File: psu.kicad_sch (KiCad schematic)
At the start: 10 parts, among them U2 TP6841

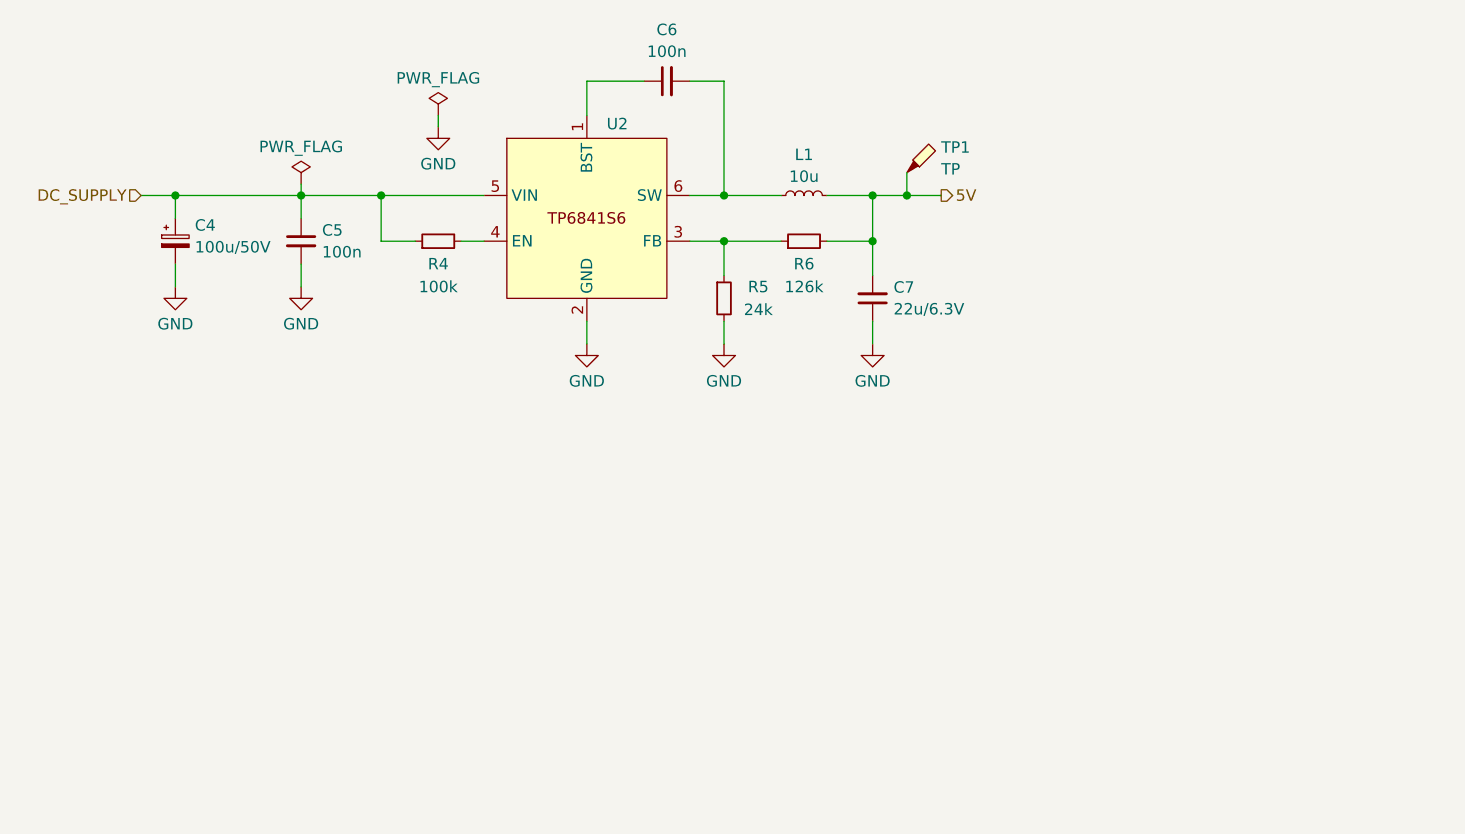
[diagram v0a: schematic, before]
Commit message: WIP PCB layout
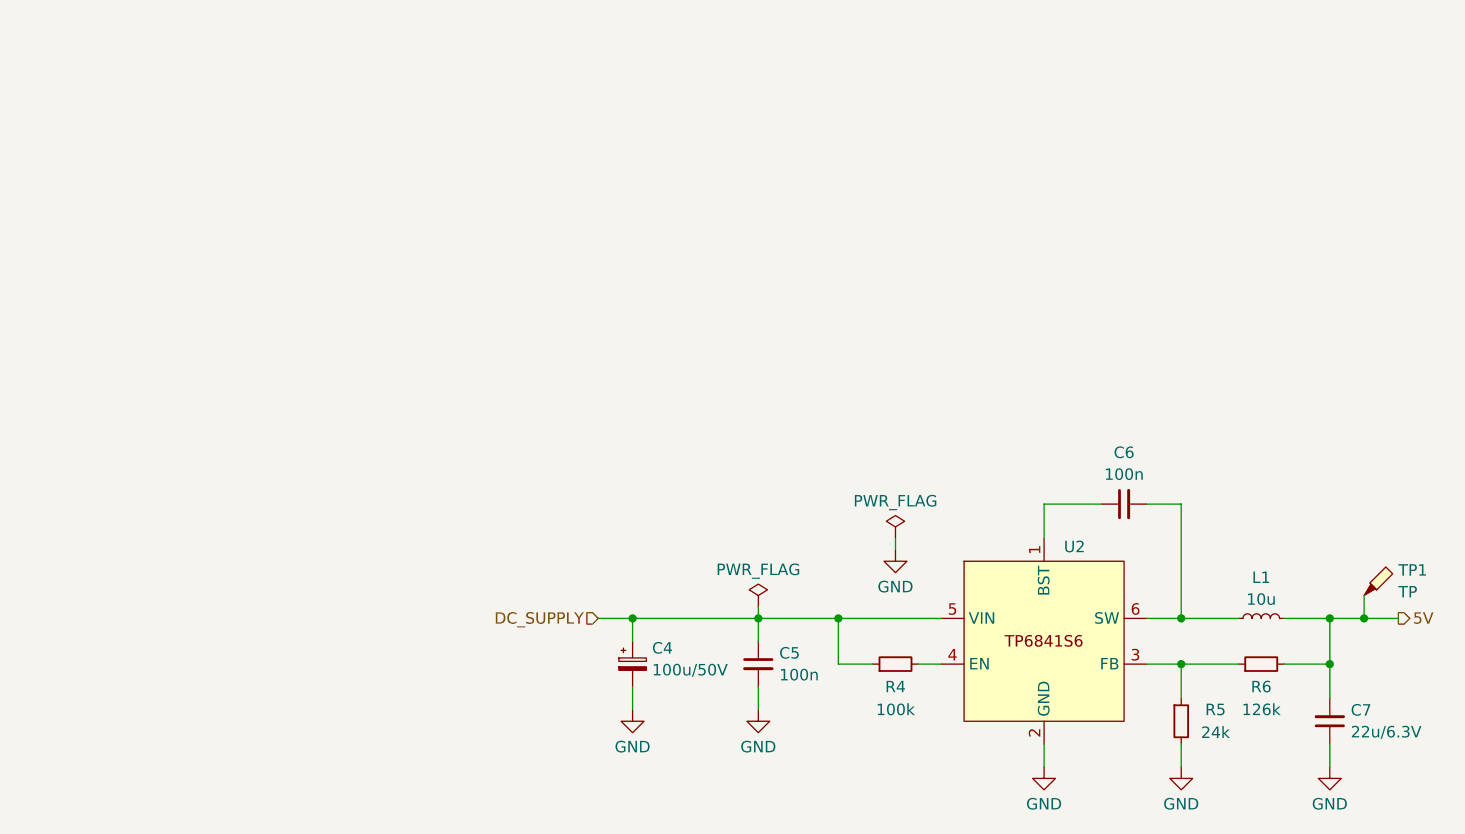
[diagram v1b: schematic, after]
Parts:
- TP1: now left out of the parts list
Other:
- company: (none) -> M17 Project
- title: (none) -> RRU CM4 board
- moved on the sheet: C4, C5, C6, C7, L1, R4, R5, R6, TP1, U2
